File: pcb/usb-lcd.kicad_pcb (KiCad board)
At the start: 2 copper layers, 41.3 x 25.5 mm, 12 parts, among them J1 USB, J2 Conn_01x02_Pin, U1 CH341A-EPP/MEM, Y1 12M

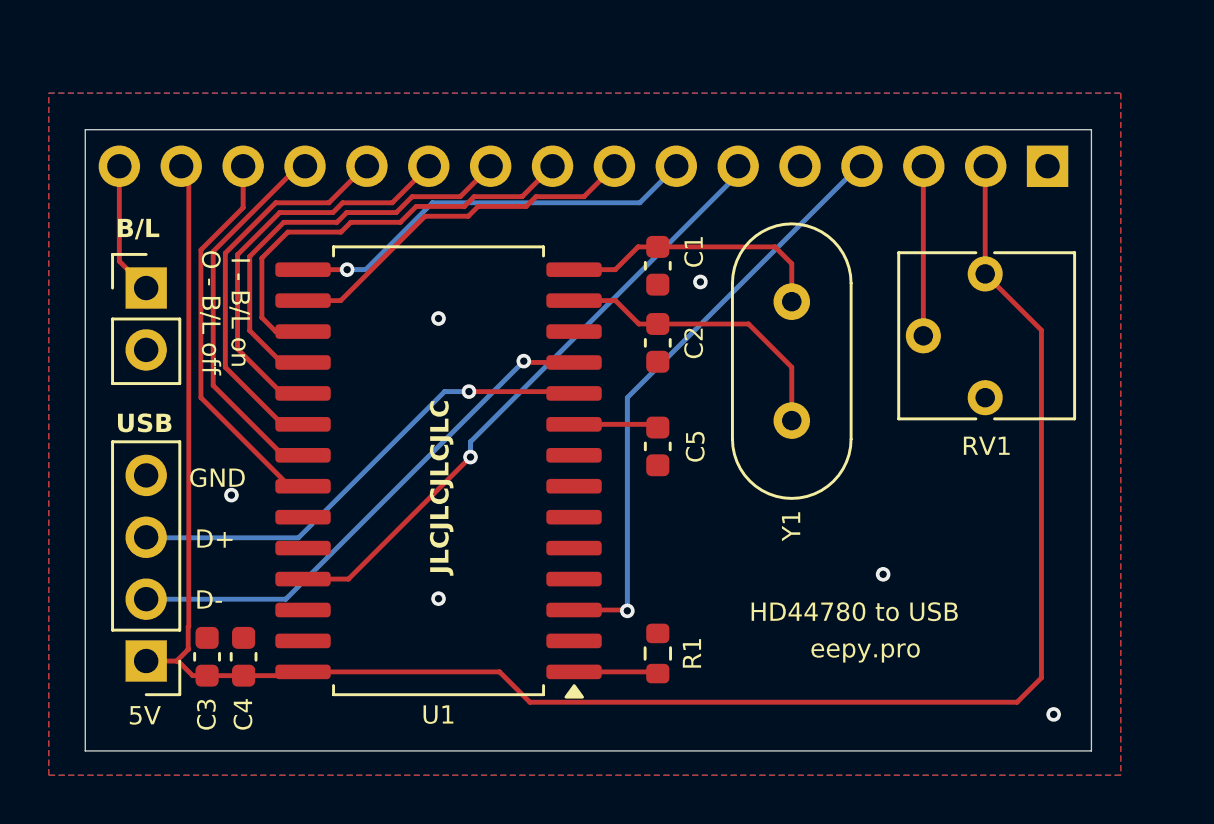
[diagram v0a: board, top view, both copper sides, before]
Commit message: Update PCB
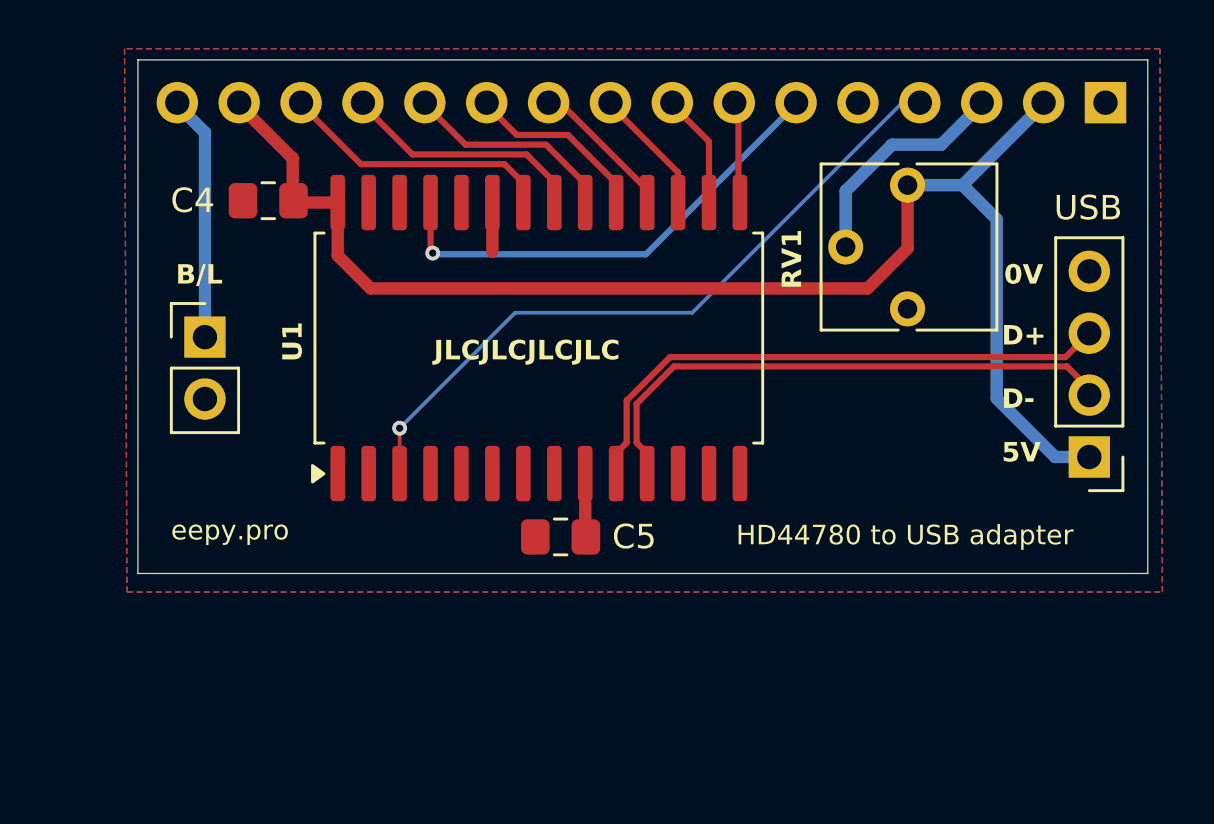
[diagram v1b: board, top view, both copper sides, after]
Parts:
- removed C1: 15pF, Capacitor_SMD:C_0603_1608Metric
- removed C2: 15p, Capacitor_SMD:C_0603_1608Metric
- removed C3: 22u, Capacitor_SMD:C_0603_1608Metric
- removed DS1: WC1602A, Connector_PinHeader_2.54mm:PinHeader_1x16_P2.54mm_Vertical
- removed R1: 2k2, Resistor_SMD:R_0603_1608Metric
- removed Y1: 12M, Crystal:Crystal_HC49-4H_Vertical
- added J3: LCD, Connector_PinHeader_2.54mm:PinHeader_1x16_P2.54mm_Vertical, B.Cu at (122.1, 54.7)
- C4, C5: footprint Capacitor_SMD:C_0603_1608Metric -> Capacitor_SMD:C_0805_2012Metric_Pad1.18x1.45mm_HandSolder
- J2: value Conn_01x02_Pin -> B/L
- U1: value CH341A-EPP/MEM -> CH341B-EPP/MEM
- moved J1 39.6 mm to (121.4, 69.2)
- moved C4 18.7 mm to (87.7, 58.7), turned to 180 degrees
- moved U1 6.83 mm to (98.8, 64.3), turned to 90 degrees
- moved C5 5.45 mm to (99.7, 72.5), turned to 180 degrees
- moved RV1 4.84 mm to (113.9, 58.1)
- moved J2 3.14 mm to (85.1, 64.3)
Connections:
- U1 pad 1: Net-(U1-ACT#) -> unconnected-(U1-ACT#-Pad1)
- U1 pad 13: Net-(U1-X1) -> GND
- U1 pad 14: Net-(U1-X0) -> unconnected-(U1-X0-Pad14)
- U1 pad 23: unconnected-(U1-SDA-Pad23) -> GND
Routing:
- net +5V: track 80.6 -> 57.2 mm
- net Net-(J3-D2): track 17.9 -> 5.18 mm
- net Net-(J3-D0): track 17.1 -> 4.49 mm, vias 1 -> 0
- net Net-(U1-X1): track 12.2 -> 0.00 mm
- net Net-(U1-X0): track 11.2 -> 0.00 mm
- net Net-(J3-D1): track 15.1 -> 4.65 mm
- net Net-(J3-D3): track 17.2 -> 8.11 mm
- net Net-(J3-D4): track 16.7 -> 9.56 mm
- net Net-(J3-E): track 25.4 -> 19.5 mm
- net Net-(J3-D5): track 16.3 -> 10.6 mm
- net /D+: track 20.1 -> 25.4 mm, vias 1 -> 0
- net Net-(J2-Pin_1): track 5.46 -> 10.0 mm
- net Net-(J3-RS): track 24.5 -> 28.7 mm
- net Net-(J3-D6): track 15.7 -> 11.9 mm
- net Net-(J3-D7): track 15.9 -> 12.3 mm
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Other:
- board size 41.3 x 25.5 mm -> 41.5 x 21.1 mm
- board text added: "0V"
- board text added: "HD44780 to USB adapter"
- board text removed: "GND"
- board text removed: "HD44780 to USB"
- board text removed: "I - B/L on O - B/L off"
- board text removed: "USB"
